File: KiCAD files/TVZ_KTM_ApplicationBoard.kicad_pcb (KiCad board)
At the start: 2 copper layers, 186 x 63.6 mm, 84 parts, among them SW1 EG1271A, SW2 EG1271A, SW3 EG1271A, SW4 EG1271A, U1 LM75B, U2 MCP2551-I-P, U3 MCP2551-I-P, U4 NUCLEO64-F446RE, U5 NUCLEO64-F446RE

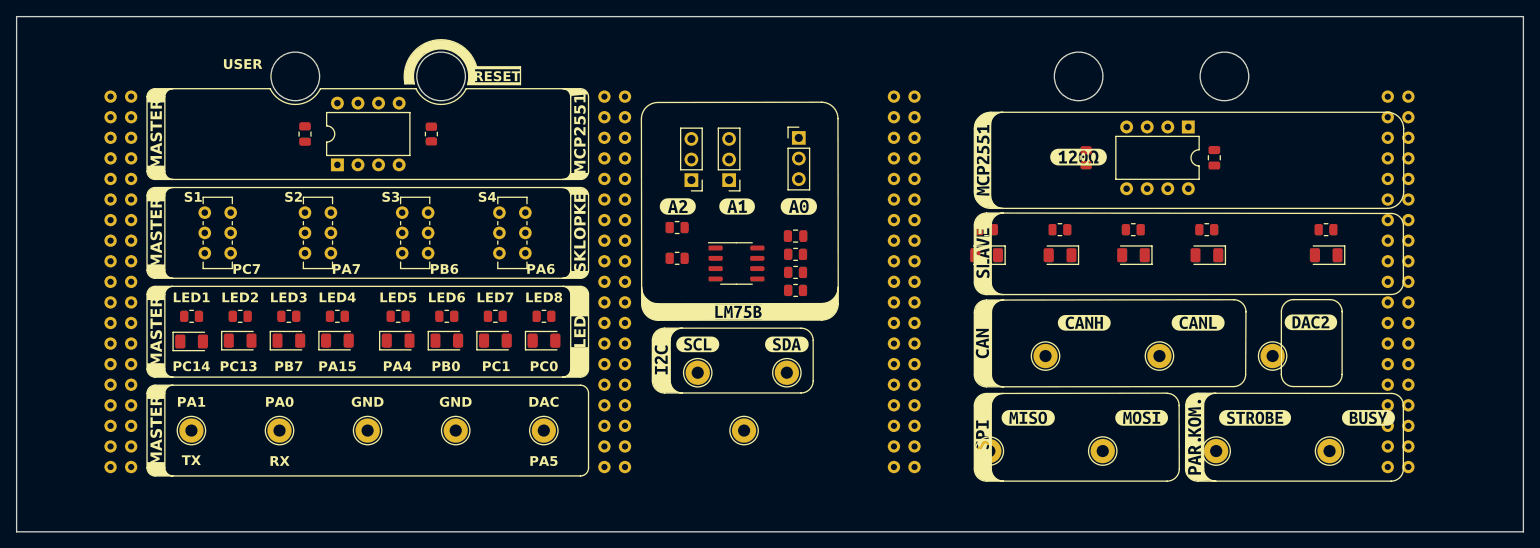
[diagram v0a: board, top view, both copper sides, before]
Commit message: update
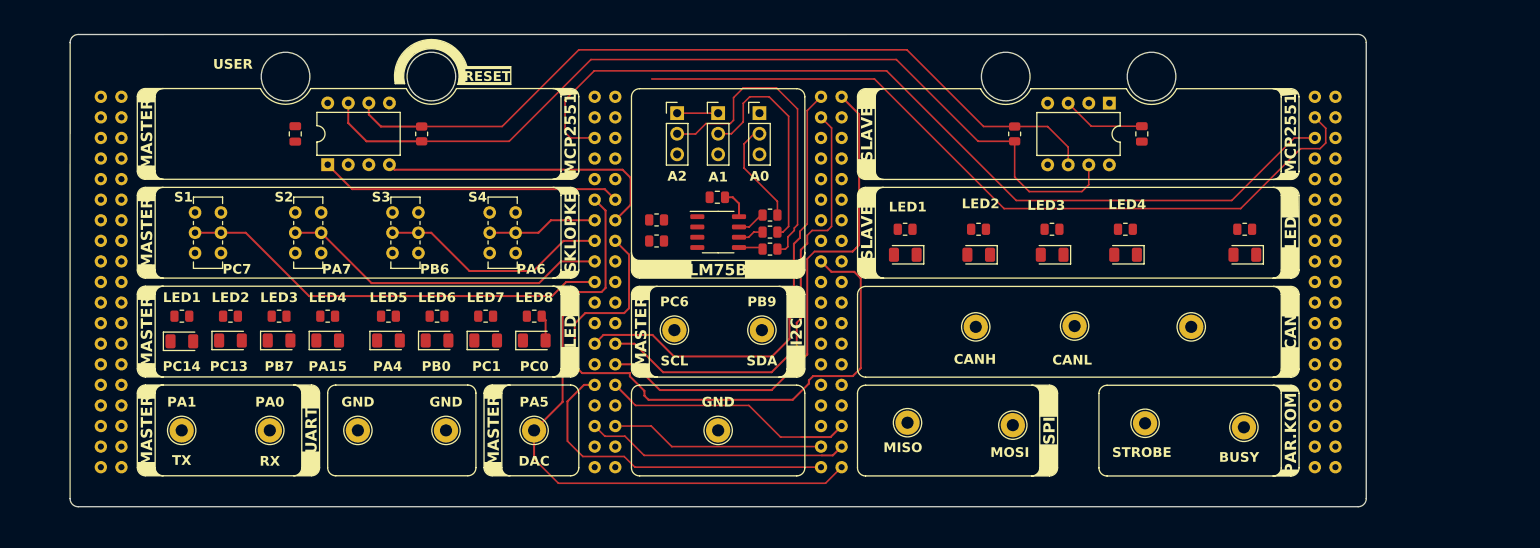
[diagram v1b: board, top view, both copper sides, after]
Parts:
- removed kibuzzard-63D0FB98: G***, kibuzzard-63D0FB98
- removed kibuzzard-63D0FBA8: G***, kibuzzard-63D0FBA8
- removed kibuzzard-63D0FCA0: G***, kibuzzard-63D0FCA0
- removed kibuzzard-63D0FCA9: G***, kibuzzard-63D0FCA9
- removed kibuzzard-63D121CA: G***, kibuzzard-63D121CA
- removed kibuzzard-63D12226: G***, kibuzzard-63D12226
- removed kibuzzard-63D12234: G***, kibuzzard-63D12234
- removed kibuzzard-63D1223E: G***, kibuzzard-63D1223E
- removed kibuzzard-63D123B4: G***, kibuzzard-63D123B4
- removed kibuzzard-63D255AB: G***, kibuzzard-63D255AB
- removed kibuzzard-63D25AA1: G***, kibuzzard-63D25AA1
- removed kibuzzard-63D26251: G***, kibuzzard-63D26251
- removed kibuzzard-63D26411: G***, kibuzzard-63D26411
- removed kibuzzard-63D26434: G***, kibuzzard-63D26434
- removed kibuzzard-63D2644E: G***, kibuzzard-63D2644E
- removed kibuzzard-63D26457: G***, kibuzzard-63D26457
- removed kibuzzard-63E0EC18: G***, kibuzzard-63E0EC18
- removed kibuzzard-63E0EE4D: G***, kibuzzard-63E0EE4D
- removed kibuzzard-63E123CE: G***, kibuzzard-63E123CE
- removed kibuzzard-63E123D9: G***, kibuzzard-63E123D9
- removed kibuzzard-648ABAA6: G***, kibuzzard-648ABAA6
- moved TP13 11.6 mm to (155.0, 77.6)
- moved TP4 11.1 mm to (162.6, 65.4)
- moved TP10 11.0 mm to (183.5, 77.9)
- moved C1 10.8 mm to (118.5, 49.5), turned to 180 degrees
- moved TP12 10.7 mm to (142.0, 77.3)
- moved TP14 10.7 mm to (177.0, 65.5)
- moved U3 10.2 mm to (166.9, 37.9)
- moved D1 10.0 mm to (141.7, 56.6)
- moved D13 10.0 mm to (183.6, 56.6)
- moved D3 10.0 mm to (159.8, 56.6)
- moved D4 10.0 mm to (168.9, 56.6)
- moved R20 10.0 mm to (183.6, 53.5)
- moved R7 10.0 mm to (150.7, 53.5)
- moved R8 10.0 mm to (159.8, 53.5)
- moved D2 10.0 mm to (150.8, 56.6)
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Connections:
- TP5 pad 1: I2C_SCL -> I2C_SDA
- TP6 pad 1: I2C_SDA -> I2C_SCL
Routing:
- net I2C_SDA: track 0.00 -> 111.8 mm
- net /CANH: track 0.00 -> 111.1 mm
- net /CANL: track 0.00 -> 99.5 mm
- net I2C_SCL: track 0.00 -> 96.9 mm
- net SPI_~{CS}: track 0.00 -> 78.0 mm
- net DAC(M)>>ADC(S): track 0.00 -> 77.9 mm
- net SPI_MISO: track 0.00 -> 65.1 mm
- net SPI_SCK: track 0.00 -> 58.0 mm
- net SPI_MOSI: track 0.00 -> 56.9 mm
- net S1: track 0.00 -> 53.3 mm
- net D1: track 0.00 -> 41.7 mm
- net S3: track 0.00 -> 40.6 mm
- net Net-(JP3-C): track 0.00 -> 38.8 mm
- net CAN_TD(M): track 0.00 -> 37.3 mm
- net CAN_RD(M): track 0.00 -> 36.5 mm
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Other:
- board size 186 x 63.6 mm -> 160 x 58.3 mm
- board text added: "A0"
- board text added: "A1"
- board text added: "A2"
- board text added: "BUSY"
- board text added: "CAN"
- board text added: "CANH"
- board text added: "CANL"
- board text added: "I2C"
- board text added: "LM75B"
- board text added: "MISO"
- board text added: "MOSI"
- board text added: "PAR.KOM."
- board text added: "PB9"
- board text added: "PC6"
- board text added: "SCL"
- board text added: "SDA"
- board text added: "SLAVE"
- board text added: "SPI"
- board text added: "STROBE"
- board text added: "UART"
